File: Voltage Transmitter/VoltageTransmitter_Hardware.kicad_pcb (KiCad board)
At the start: 2 copper layers, 30.5 x 71.9 mm, 8 parts, among them U1 OKI, U2 ESP8266_MCU

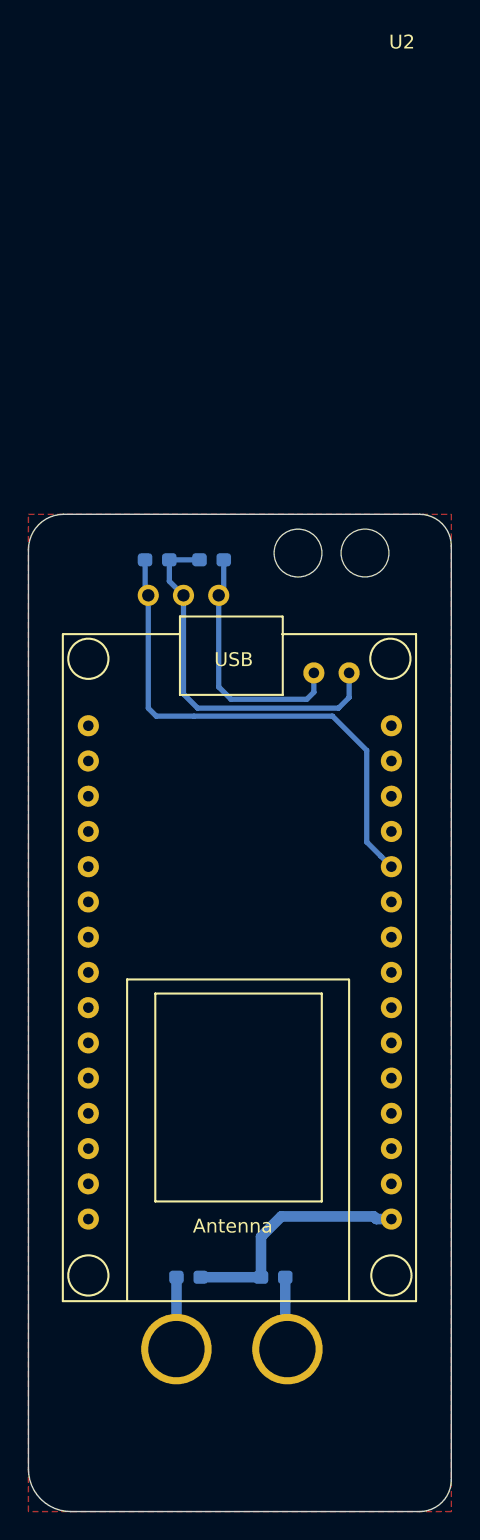
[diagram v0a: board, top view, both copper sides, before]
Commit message: Gerbs Made
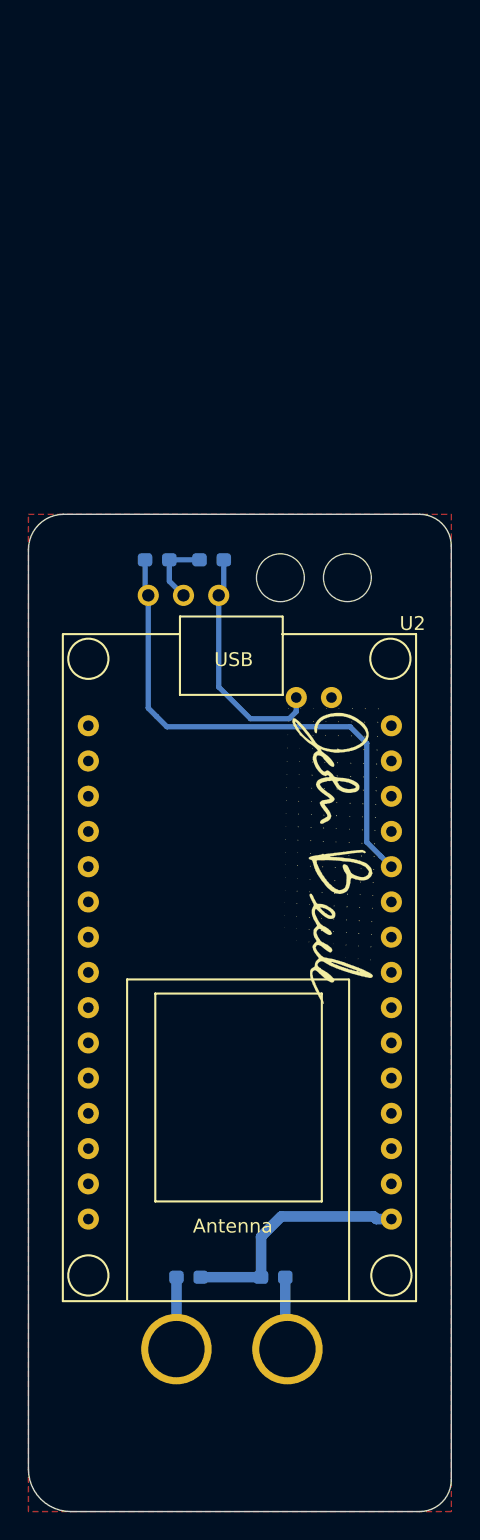
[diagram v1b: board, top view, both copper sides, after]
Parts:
- added G***: LOGO, Voltage_Transmitter_Hardware:Austin_Christman_22mmX8.3mm, B.Cu at (127.3, 80.8)
- added G***: LOGO, Voltage_Transmitter_Hardware:John_Beuke_22mmX7.4mm, F.Cu at (138.7, 73.2)
- moved Conn2 2.18 mm to (137.4, 61.7)
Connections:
- C1 pad 2: Net-(C1-Pad2) -> GND
- C2 pad 2: Net-(C1-Pad2) -> GND
- Conn2 pad 1: Net-(C1-Pad2) -> GND
- U1 pad 2: Net-(C1-Pad2) -> GND
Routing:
- net Net-(C1-Pad2): track 26.7 -> 0.00 mm
- net GND: track 5.18 -> 10.3 mm
- net Net-(C1-Pad1): track 18.1 -> 17.1 mm
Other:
- board text added: "Voltage Transmitter, Rev 1 Mars Rover Design Team Missouri S&T, 2019 Austin Christman, John Beuke"
- board text removed: "Voltage Transmitter, Rev 1 Mars Rover Design Team Missouri S&T Austin Christman, John Beuke"
